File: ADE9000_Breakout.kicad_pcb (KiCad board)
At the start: 2 copper layers, 38.1 x 27.9 mm, 58 parts, among them J1 PWR, J2 Current In, J3 Voltage In, U1 ADE9000, Y1 24.576MHz

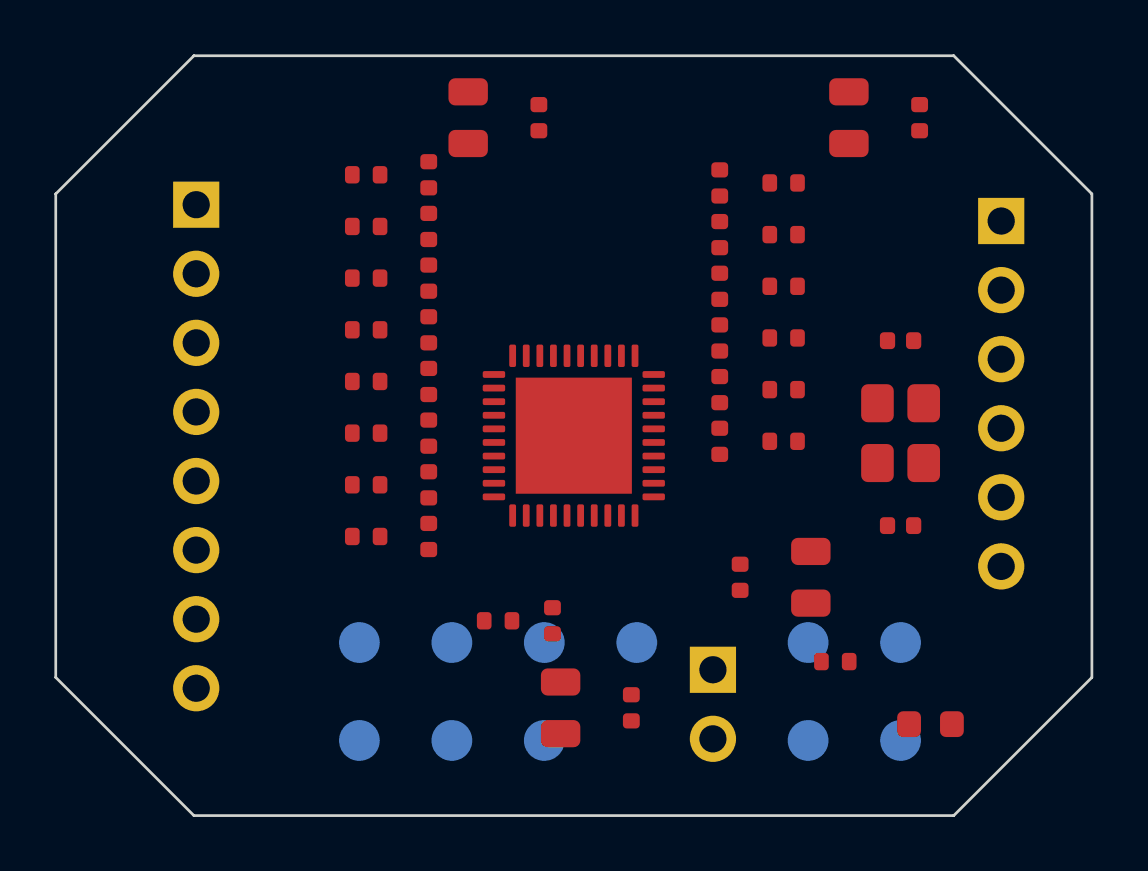
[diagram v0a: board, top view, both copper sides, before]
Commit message: Complete routing
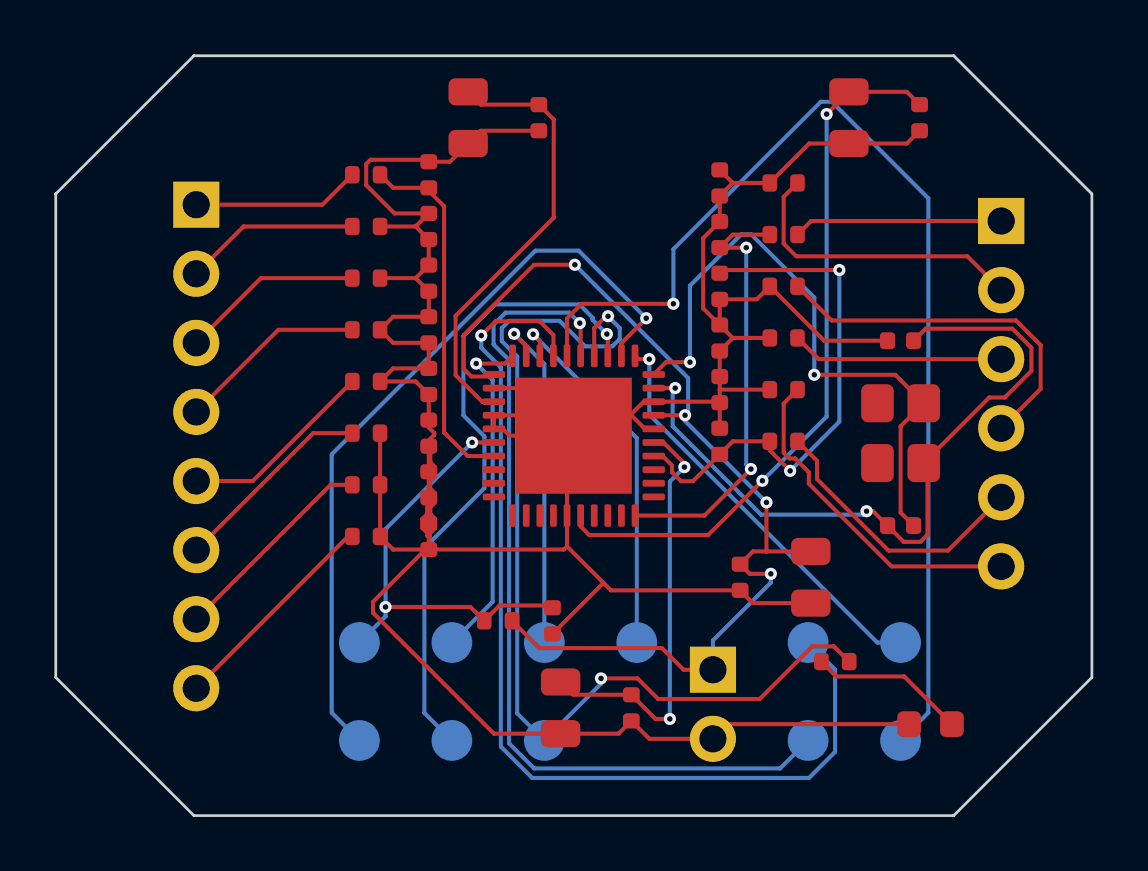
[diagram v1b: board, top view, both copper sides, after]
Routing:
- net GND: track 0.00 -> 134.6 mm
- net CF4_DREADY: track 0.00 -> 41.0 mm, vias 0 -> 1
- net +3V3: track 0.00 -> 39.0 mm, vias 0 -> 4
- net CF2: track 0.00 -> 37.1 mm, vias 0 -> 2
- net SCLK: track 0.00 -> 36.9 mm, vias 0 -> 1
- net CF3_ZX: track 0.00 -> 32.2 mm, vias 0 -> 1
- net IRQ1: track 0.00 -> 28.4 mm, vias 0 -> 1
- net CLKIN: track 0.00 -> 27.3 mm, vias 0 -> 2
- net REF: track 0.00 -> 26.5 mm, vias 0 -> 2
- net CF1: track 0.00 -> 23.6 mm, vias 0 -> 1
- net CLKOUT: track 0.00 -> 23.0 mm, vias 0 -> 2
- net VCP: track 0.00 -> 19.4 mm, vias 0 -> 2
- net RESET: track 0.00 -> 16.5 mm, vias 0 -> 2
- net DVDDOUT: track 0.00 -> 16.3 mm
- net VAP: track 0.00 -> 16.2 mm, vias 0 -> 2
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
